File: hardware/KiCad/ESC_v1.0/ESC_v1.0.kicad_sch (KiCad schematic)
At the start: 159 parts, among them J1 Conn_01x03_Socket, J2 Conn_01x03_Socket, J3 Conn_ARM_SWD_TagConnect_TC203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, Q1 NVMFS5C604N, Q2 NVMFS5C604N, Q3 NVMFS5C604N, Q4 NVMFS5C604N, Q5 NVMFS5C604N, Q6 NVMFS5C604N, U1 STM32G484CEU6, U2 LM5160A, U3 TPS7B92033, U4 2EDL8024, U5 2EDL8024, U6 2EDL8024, X1 16MHz

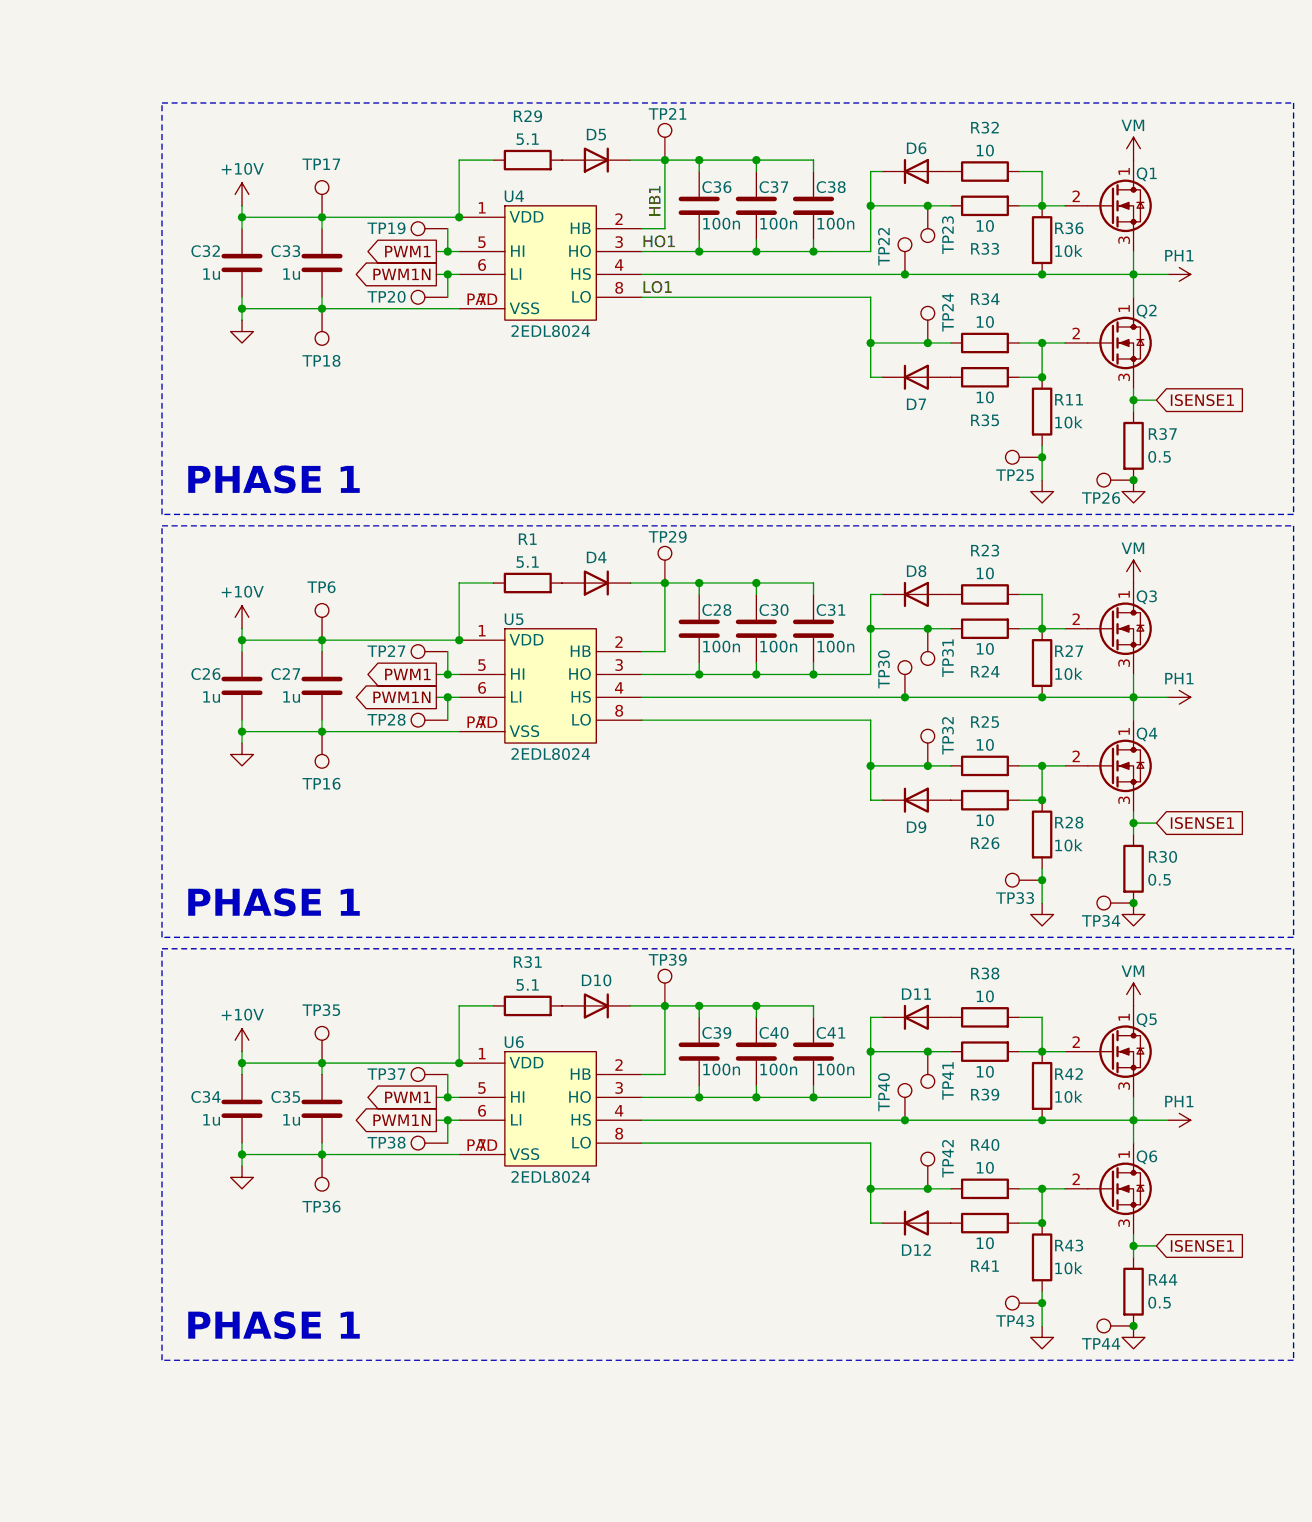
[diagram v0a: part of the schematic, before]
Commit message: Kicad and esc choice review
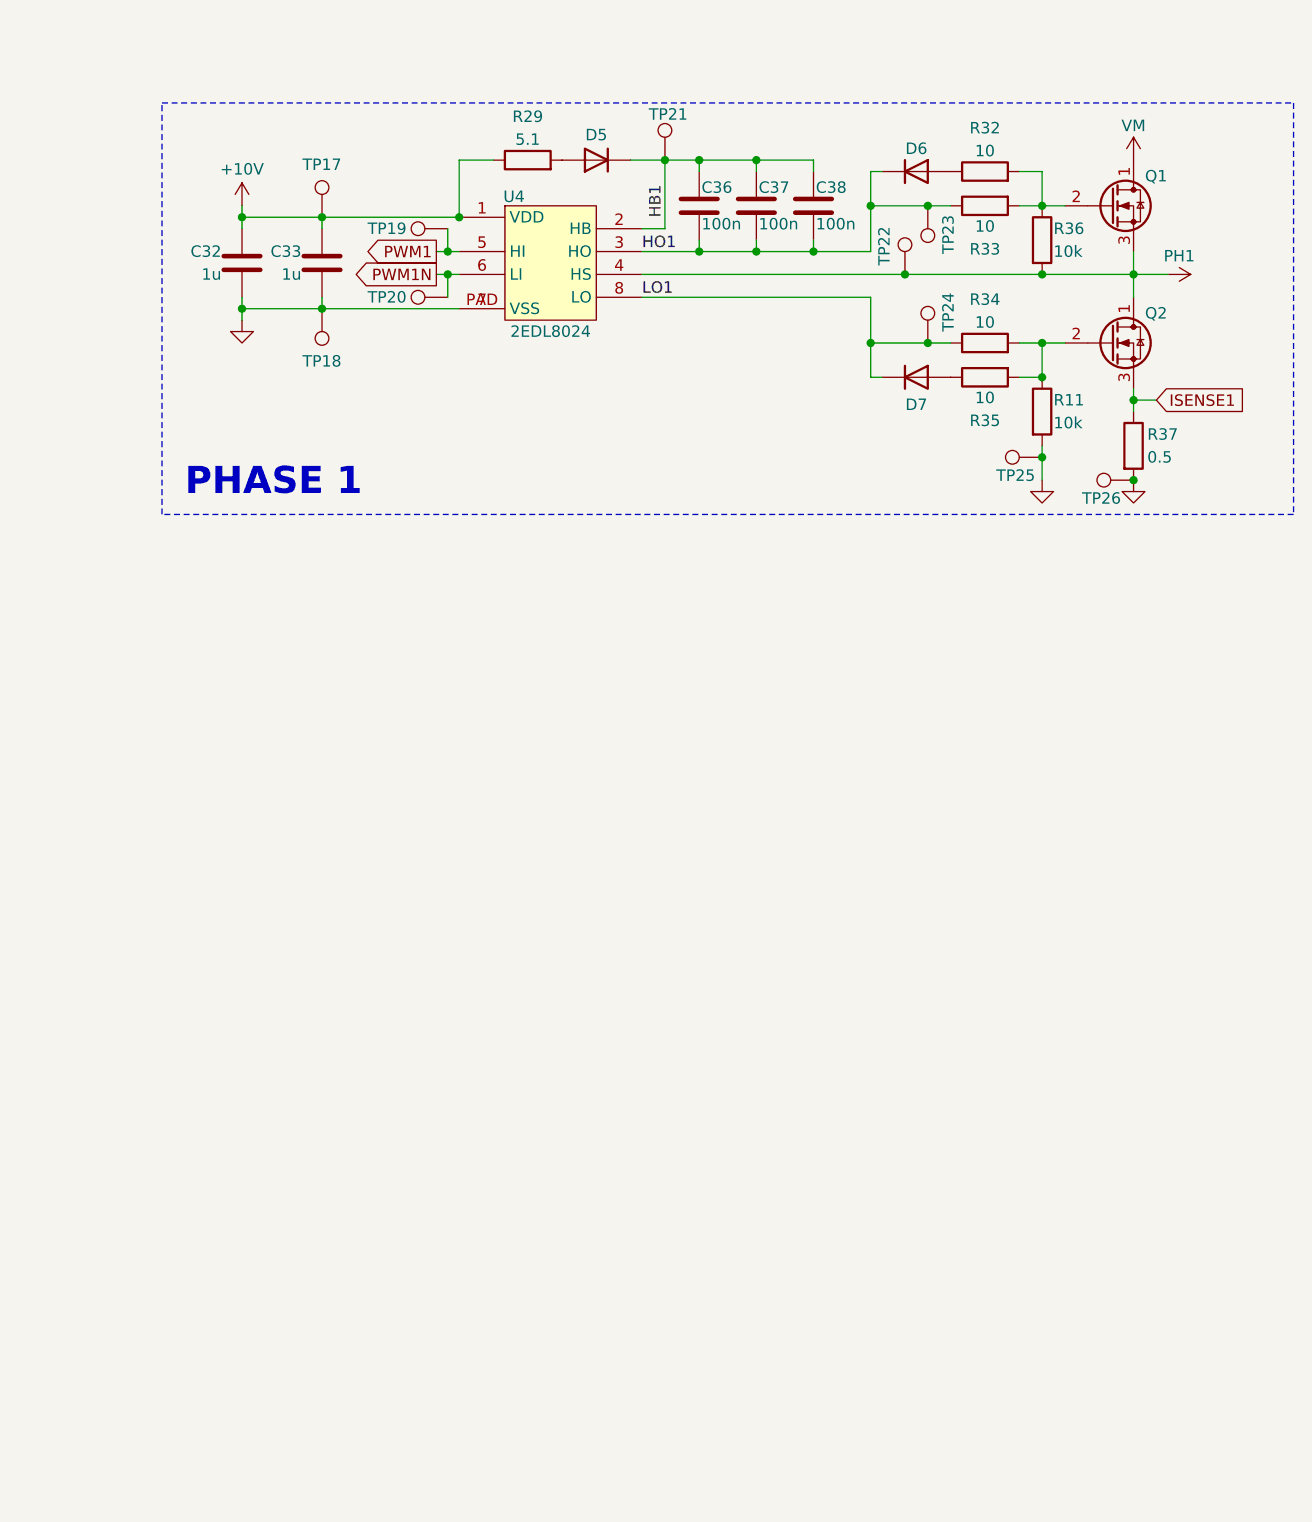
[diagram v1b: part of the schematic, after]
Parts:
- removed C26, C27, C34, C35: 1u, Capacitor_SMD:C_0603_1608Metric, symbol ESC-SchemSymLib:CL10A105KB8NNNC
- removed C28, C30, C31, C39, C40, C41: 100n, Capacitor_SMD:C_0402_1005Metric, symbol ESC-SchemSymLib:CL05B104KO5NNNC
- removed D10, D11, D12, D4, D8, D9: RB161QS-40T18R, ESC-FootprintLib:Rohm_SMD1006, symbol ESC-SchemSymLib:RB161QS-40T18R
- removed Q1, Q2, Q3, Q4, Q5, Q6: NVMFS5C604N, ESC-FootprintLib:Onsemi_DFN5_DFNW5, symbol ESC-SchemSymLib:NVMFS5C604NL
- removed R1, R31: 5.1, Resistor_SMD:R_0805_2012Metric, symbol ESC-SchemSymLib:0805W8F510KT5E
- removed R23, R24, R25, R26, R38, R39, R40, R41: 10, Resistor_SMD:R_0805_2012Metric, symbol ESC-SchemSymLib:0805W8F100JT5E
- removed R27, R28, R42, R43: 10k, Resistor_SMD:R_0603_1608Metric, symbol ESC-SchemSymLib:0603WAF1002T5E
- removed R30, R44: 0.5, ESC-FootprintLib:Kelvin Shunt 1216 (3038), symbol ESC-SchemSymLib:HoBB1216-5W-0.5mR-1%
- removed TP16, TP27, TP28, TP29, TP30, TP31, TP32, TP33, TP34, TP35, TP36, TP37, TP38, TP39, TP40, TP41, TP42, TP43, TP44, TP6: TestPoint, symbol Connector:TestPoint
- removed U5, U6: 2EDL8024, Package_DFN_QFN:DFN-8-1EP_4x4mm_P0.8mm_EP2.5x3.6mm, symbol ESC-SchemSymLib:2EDL8024
- added Q1, Q2: CSD18540Q5B, ESC-FootprintLib:TRANS_CSD18540Q5B, symbol ESC-SchemSymLib:CSD18540Q5B
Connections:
- net ISENSE1: now also Q2.3 (S)
- net PH1: now also Q1.3 (S), Q2.1 (D)
- net VM: now also Q1.1 (D)
- net at R11.1, R34.2, R35.2: now also Q2.2 (G)
- net at R32.2, R33.2, R36.1: now also Q1.2 (G)
